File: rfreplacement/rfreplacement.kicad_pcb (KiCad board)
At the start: 2 copper layers, 43.9 x 55.9 mm, 27 parts

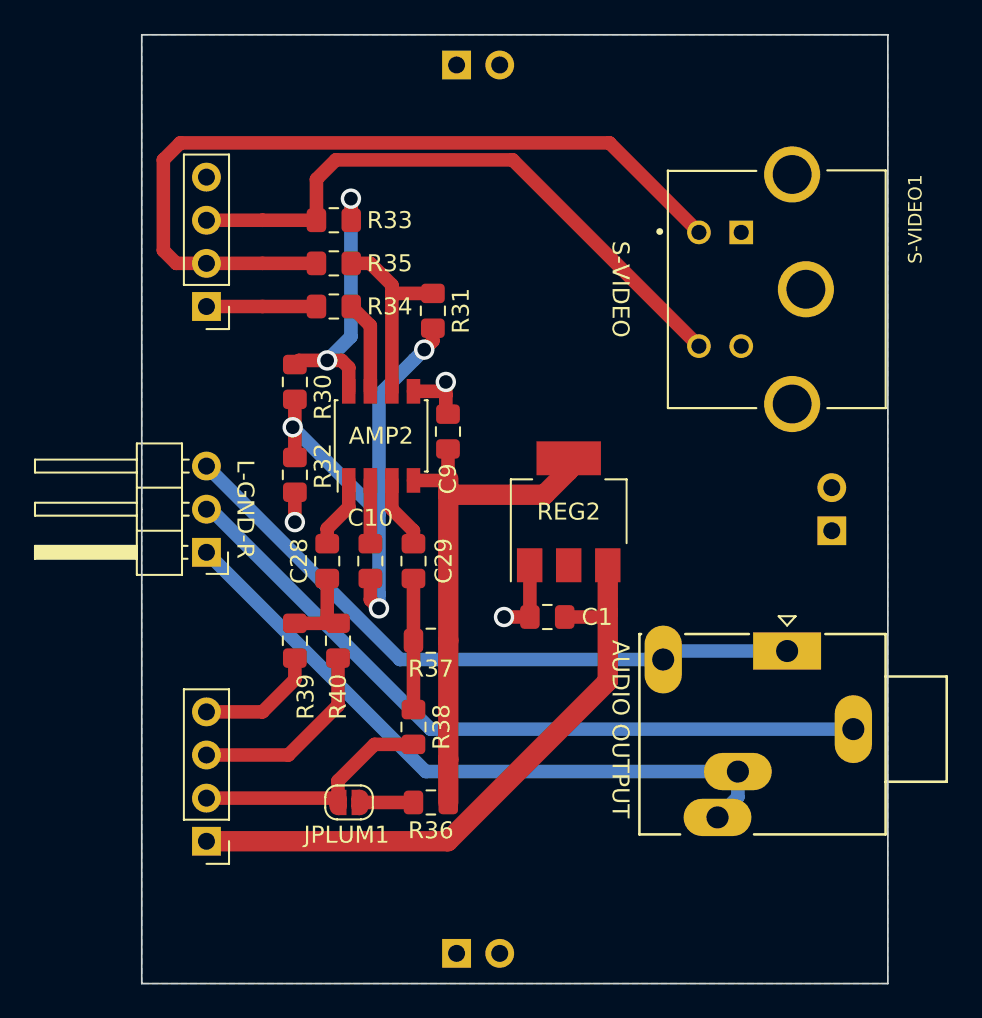
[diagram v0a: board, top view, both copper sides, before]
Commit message: Layout cleanup.
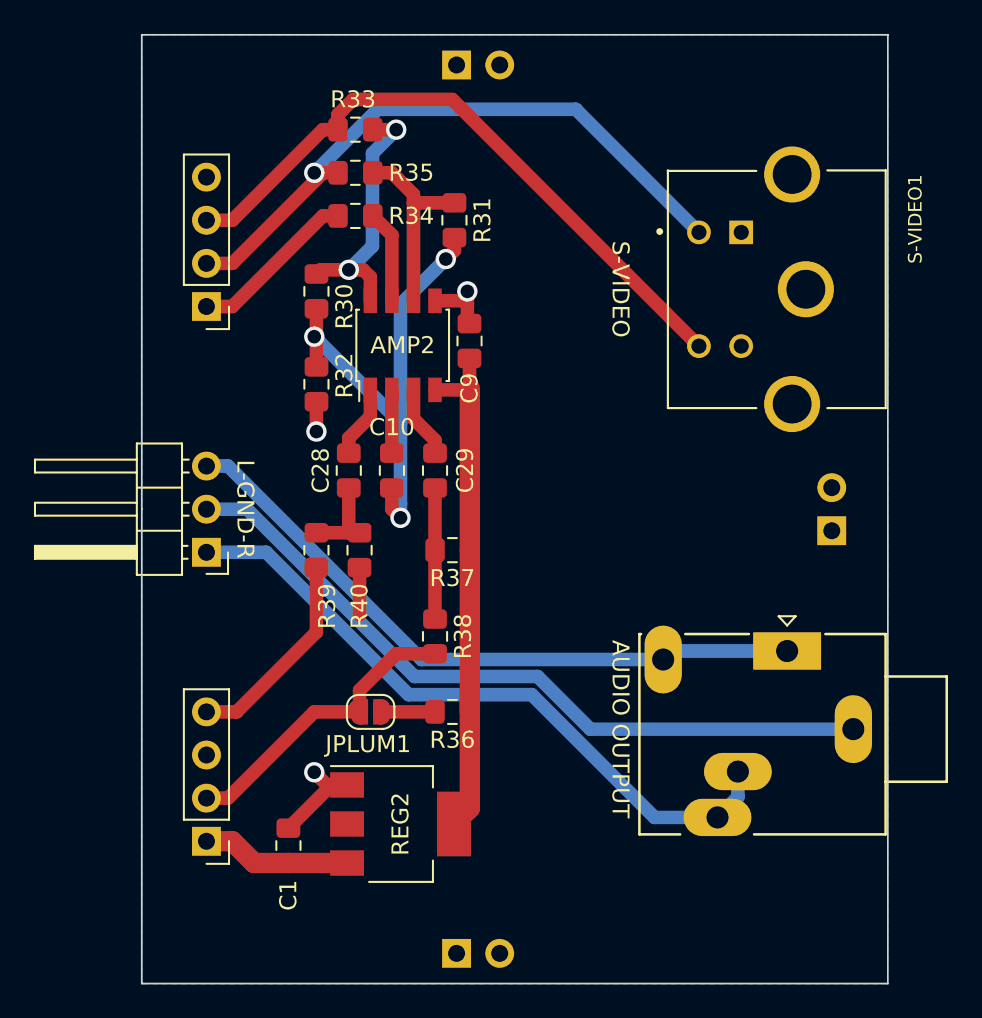
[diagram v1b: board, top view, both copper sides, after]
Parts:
- moved REG2 20.9 mm to (119.4, 101.6), turned to 0 degrees
- moved C1 20.3 mm to (112.8, 102.9), turned to 270 degrees
- moved JPLUM1 5.48 mm to (117.6, 95.0)
- moved R30 5.48 mm to (114.4, 70.2)
- moved R32 5.48 mm to (114.4, 75.7)
- moved R38 5.48 mm to (121.4, 90.6)
- moved R39 5.48 mm to (114.4, 85.5)
- moved C9 5.48 mm to (123.4, 73.2)
- moved R33 5.48 mm to (116.7, 60.7)
- moved R34 5.48 mm to (116.7, 65.8)
- moved R36 5.48 mm to (122.4, 95.0)
- moved R37 5.48 mm to (122.4, 85.5)
- moved R40 5.48 mm to (117.0, 85.5)
- moved R35 5.48 mm to (116.7, 63.2)
- moved AMP2 5.48 mm to (119.5, 73.4)
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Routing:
- net +12V: track 37.0 -> 8.81 mm
- net /LUMA_OUT: track 48.8 -> 37.2 mm, vias 0 -> 1
- net GNDA: track 22.0 -> 14.3 mm
- net /CHROMA_IN: track 7.26 -> 12.2 mm
- net /LUMA_IN: track 14.5 -> 18.1 mm
- net /COMPOSITE_OUT: track 6.48 -> 9.96 mm
- net /CHROMA_OUT: track 36.4 -> 38.5 mm
- net Net-(AMP2-Pad8): track 16.2 -> 15.6 mm
